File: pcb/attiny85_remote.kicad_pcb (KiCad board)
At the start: 2 copper layers, 24.2 x 70 mm, 29 parts, among them J1 RST/DRV, J2 INT/DRV, J3 PWR, Q1 SSM3J35AFS,LF, SW1 F2, SW2 F2, SW3 F2, U1 Ra-02

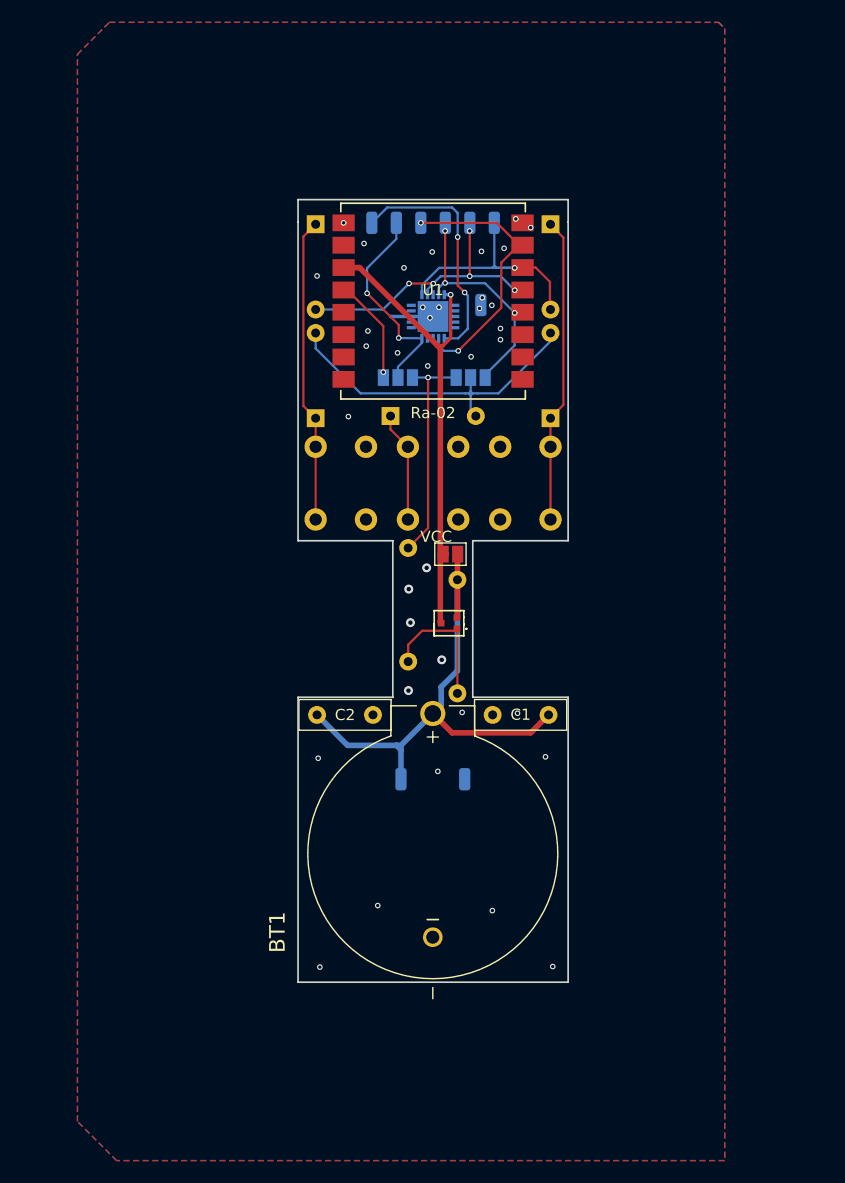
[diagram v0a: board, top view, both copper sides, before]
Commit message: kikit tabs
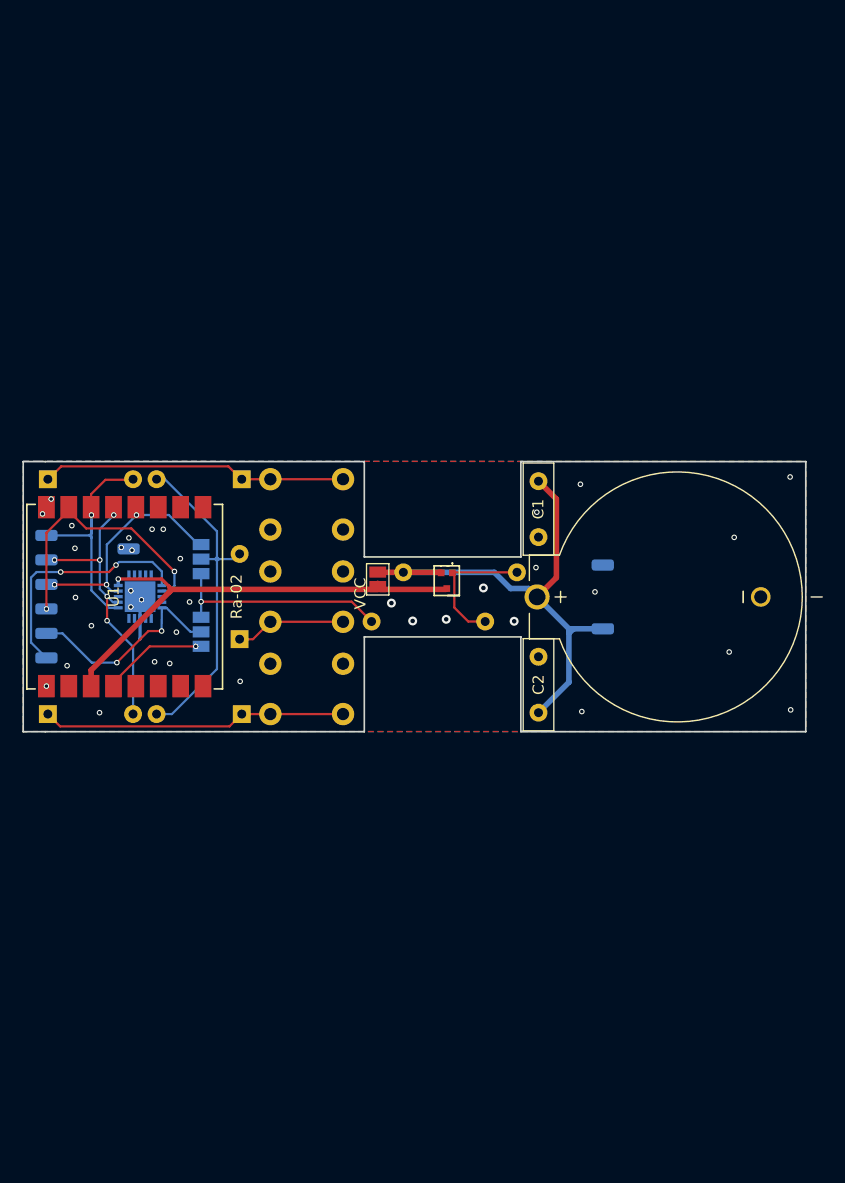
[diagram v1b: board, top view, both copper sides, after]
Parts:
- added REF**: Tab, kikit:Tab, F.Cu at (211.7, 67.6)
- added REF**: Tab, kikit:Tab, F.Cu at (224.7, 80.0)
- added REF**: Tab, kikit:Tab, F.Cu at (154.2, 80.0)
- added REF**: Tab, kikit:Tab, F.Cu at (211.7, 92.3)
- added REF**: Tab, kikit:Tab, F.Cu at (170.7, 92.3)
- added REF**: Tab, kikit:Tab, F.Cu at (170.7, 67.6)
- moved D6 50.4 mm to (156.7, 69.5), turned to 0 degrees
- moved D4 49.9 mm to (156.7, 90.5), turned to 0 degrees
- moved REF** 48.8 mm to (156.5, 74.5), turned to -90 degrees
- moved REF** 48.6 mm to (156.5, 85.4), turned to -90 degrees
- moved REF** 48.4 mm to (156.5, 76.7), turned to -90 degrees
- moved REF** 48.2 mm to (156.5, 83.2), turned to -90 degrees
- moved REF** 48.1 mm to (156.5, 78.9), turned to -90 degrees
- moved REF** 48.1 mm to (156.5, 81.0), turned to -90 degrees
- moved REF** 38.3 mm to (163.9, 75.7), turned to -90 degrees
- moved U1 38.2 mm to (163.5, 80.0), turned to 90 degrees
- moved G*** 37.6 mm to (216.8, 84.6), turned to -90 degrees
- moved Attiny85 36.2 mm to (164.9, 80.0), turned to 180 degrees
- moved J2 29.1 mm to (170.4, 76.6), turned to 90 degrees
- moved J1 28.8 mm to (170.4, 83.1), turned to -90 degrees
- moved D5 28.1 mm to (174.0, 69.5), turned to 180 degrees
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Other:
- board size 24.2 x 70 mm -> 70 x 24.2 mm
